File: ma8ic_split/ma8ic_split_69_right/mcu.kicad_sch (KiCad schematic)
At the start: 26 parts, among them J1 USB_C_Receptacle, J2 MJ-4PP-9, SW1 SW_PUSH, U1 ATMEGA32U4, X1 CSTNE16M0V530000R0

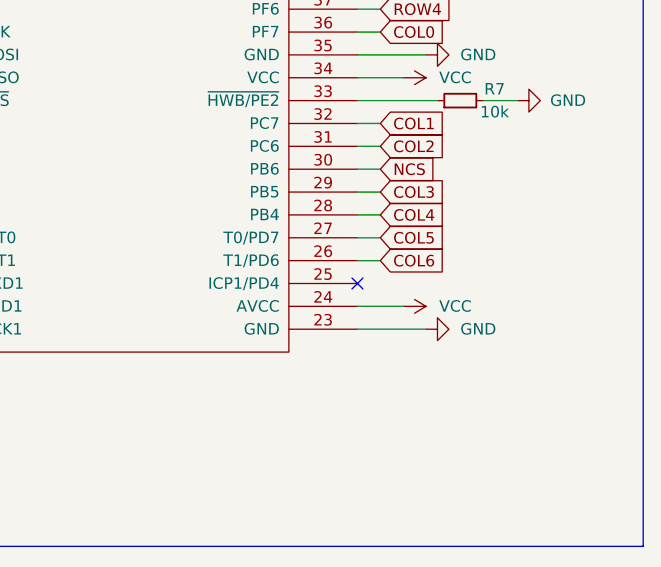
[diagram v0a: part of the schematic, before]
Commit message: update
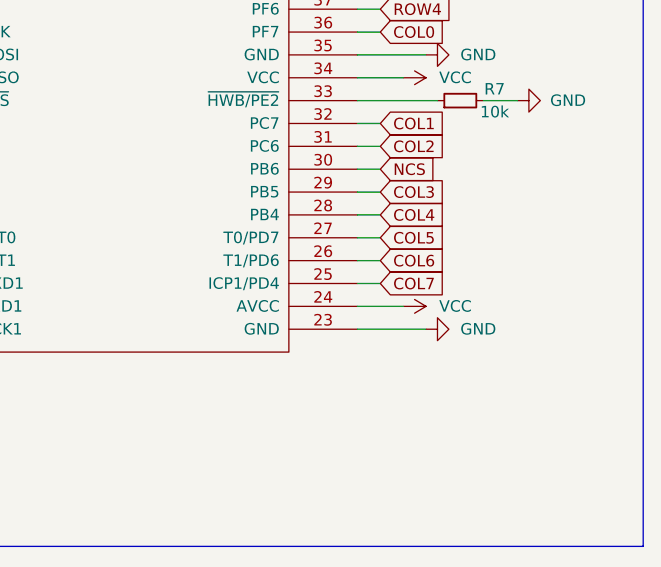
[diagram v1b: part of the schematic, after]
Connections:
- net COL7: now reaches U1.25 (ICP1/PD4)
- no-connect marks 14 -> 13
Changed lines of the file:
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@@
   (no_connect (at 52.07 66.04))
   (no_connect (at 50.8 173.99))
-  (no_connect (at 209.55 81.28))
   (no_connect (at 154.94 60.96))
   (no_connect (at 154.94 33.02))
@@
     (stroke (width 0) (type default) (color 0 0 0 0))
   )
+  (wire (pts (xy 209.55 81.28) (xy 212.09 81.28))
+    (stroke (width 0) (type default) (color 0 0 0 0))
+  )
   (wire (pts (xy 95.25 175.26) (xy 95.25 177.8))
     (stroke (width 0) (type default) (color 0 0 0 0))
@@
     (effects (font (size 1.27 1.27)) (justify right bottom))
   )
+  (global_label "COL7" (shape input) (at 212.09 81.28 0) (fields_autoplaced)
+    (effects (font (size 1.27 1.27)) (justify left))
+    (property "Intersheet References" "${INTERSHEET_REFS}" (id 0) (at 219.3412 81.2006 0)
+      (effects (font (size 1.27 1.27)) (justify left) hide)
+    )
+  )
   (global_label "ROW2" (shape input) (at 212.09 45.72 0) (fields_autoplaced)

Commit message: update
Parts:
- C1, C3, C4, C5, C6: LCSC (none) -> C14663
- C2: LCSC (none) -> C15849
- C7: LCSC (none) -> C19666
- D1, D2: LCSC (none) -> C84263
- D3: LCSC (none) -> C84266
- J1: LCSC (none) -> C778726
- R1, R2: LCSC (none) -> C23186
- R10, R11, R6, R7: LCSC (none) -> C25804
- R3, R4: LCSC (none) -> C23345
- R5, R8, R9: LCSC (none) -> C21190
- U1: footprint ma8ic_split_69:TQFP-44_10x10mm_P0.8mm -> ma8ic_split_69:QFN-44-1EP_7x7mm_P0.5mm_EP5.2x5.2mm; LCSC (none) -> C112161
- X1: LCSC (none) -> C341521
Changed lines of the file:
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@@
+      (effects (font (size 1.27 1.27)) hide)
+    )
+    (property "LCSC" "C14663" (id 4) (at 25.4 134.62 0)
       (effects (font (size 1.27 1.27)) hide)
     )
@@
       (effects (font (size 1.27 1.27)) hide)
     )
+    (property "LCSC" "C25804" (id 4) (at 138.43 58.42 0)
+      (effects (font (size 1.27 1.27)) hide)
+    )
     (pin "1")
     (pin "2")
@@
       (effects (font (size 1.27 1.27)) hide)
     )
+    (property "LCSC" "C19666" (id 4) (at 50.8 134.62 0)
+      (effects (font (size 1.27 1.27)) hide)
+    )
     (pin "1")
     (pin "2")
@@
     )
     (property "Datasheet" "~" (id 3) (at 220.98 38.1 0)
+      (effects (font (size 1.27 1.27)) hide)
+    )
+    (property "LCSC" "C14663" (id 4) (at 220.98 38.1 0)
       (effects (font (size 1.27 1.27)) hide)
     )
@@
       (effects (font (size 1.27 1.27)) (justify bottom) hide)
     )
+    (property "LCSC" "C341521" (id 8) (at 138.43 133.35 0)
+      (effects (font (size 1.27 1.27)) hide)
+    )
     (pin "1")
     (pin "2")
@@
       (effects (font (size 1.27 1.27)) hide)
     )
+    (property "LCSC" "C21190" (id 4) (at 137.16 86.36 0)
+      (effects (font (size 1.27 1.27)) hide)
+    )
     (pin "1")
     (pin "2")
@@
       (effects (font (size 1.27 1.27)) hide)
     )
+    (property "LCSC" "C23186" (id 4) (at 59.69 30.48 0)
+      (effects (font (size 1.27 1.27)) hide)
+    )
     (pin "1")
     (pin "2")
@@
       (effects (font (size 1.27 1.27)) hide)
     )
+    (property "LCSC" "C23186" (id 4) (at 59.69 33.02 0)
+      (effects (font (size 1.27 1.27)) hide)
+    )
     (pin "1")
     (pin "2")
@@
       (effects (font (size 1.27 1.27)) hide)
     )
+    (property "LCSC" "C25804" (id 4) (at 220.98 60.96 0)
+      (effects (font (size 1.27 1.27)) hide)
+    )
     (pin "1")
     (pin "2")
@@
     )
     (property "Datasheet" "https://www.usb.org/sites/default/files/documents/usb_type-c.zip" (id 3) (at 40.64 50.8 0)
+      (effects (font (size 1.27 1.27)) hide)
+    )
+    (property "LCSC" "C778726" (id 4) (at 36.83 50.8 0)
       (effects (font (size 1.27 1.27)) hide)
     )
@@
       (effects (font (size 1.27 1.27)) hide)
     )
+    (property "LCSC" "C14663" (id 4) (at 38.1 134.62 0)
+      (effects (font (size 1.27 1.27)) hide)
+    )
     (pin "1")
     (pin "2")
@@
     )
     (property "Datasheet" "~" (id 3) (at 44.45 134.62 0)
+      (effects (font (size 1.27 1.27)) hide)
+    )
+    (property "LCSC" "C14663" (id 4) (at 44.45 134.62 0)
       (effects (font (size 1.27 1.27)) hide)
     )
@@
       (effects (font (size 1.27 1.27)) hide)
     )
+    (property "LCSC" "C23345" (id 4) (at 59.69 43.18 0)
+      (effects (font (size 1.27 1.27)) hide)
+    )
     (pin "1")
     (pin "2")
@@
       (effects (font (size 1.27 1.27)) hide)
     )
+    (property "LCSC" "C21190" (id 4) (at 82.55 137.16 0)
+      (effects (font (size 1.27 1.27)) hide)
+    )
     (pin "1")
     (pin "2")
@@
       (effects (font (size 1.27 1.27)) hide)
     )
+    (property "LCSC" "C14663" (id 4) (at 31.75 134.62 0)
+      (effects (font (size 1.27 1.27)) hide)
+    )
     (pin "1")
     (pin "2")
@@
       (effects (font (size 1.27 1.27)) hide)
     )
+    (property "LCSC" "C84263" (id 4) (at 128.27 50.8 0)
+      (effects (font (size 1.27 1.27)) hide)
+    )
     (pin "1")
     (pin "2")
@@
       (effects (font (size 1.27 1.27)) hide)
     )
+    (property "LCSC" "C23345" (id 4) (at 59.69 40.64 0)
+      (effects (font (size 1.27 1.27)) hide)
+    )
     (pin "1")
     (pin "2")
@@
       (effects (font (size 1.27 1.27)) hide)
     )
+    (property "LCSC" "C25804" (id 4) (at 95.25 180.34 0)
+      (effects (font (size 1.27 1.27)) hide)
+    )
     (pin "1")
     (pin "2")
@@
       (effects (font (size 1.27 1.27)) hide)
     )
+    (property "LCSC" "C25804" (id 4) (at 88.9 180.34 0)
+      (effects (font (size 1.27 1.27)) hide)
+    )
     (pin "1")
     (pin "2")
@@
     )
     (property "Datasheet" "~" (id 3) (at 148.59 45.72 0)
+      (effects (font (size 1.27 1.27)) hide)
+    )
+    (property "LCSC" "C15849" (id 4) (at 148.59 45.72 0)
       (effects (font (size 1.27 1.27)) hide)
     )
@@
       (effects (font (size 1.27 1.27)) hide)
     )
+    (property "LCSC" "C84266" (id 4) (at 91.44 137.16 0)
+      (effects (font (size 1.27 1.27)) hide)
+    )
     (pin "1")
     (pin "2")
@@
       (effects (font (size 1.27 1.27)) hide)
     )
+    (property "LCSC" "C84263" (id 4) (at 128.27 86.36 0)
+      (effects (font (size 1.27 1.27)) hide)
+    )
     (pin "1")
     (pin "2")
@@
       (effects (font (size 1.524 1.524)))
     )
-    (property "Footprint" "ma8ic_split_69:TQFP-44_10x10mm_P0.8mm" (id 2) (at 181.61 59.69 0)
+    (property "Footprint" "ma8ic_split_69:QFN-44-1EP_7x7mm_P0.5mm_EP5.2x5.2mm" (id 2) (at 181.61 59.69 0)
       (effects (font (size 1.524 1.524)) hide)
     )
     (property "Datasheet" "" (id 3) (at 181.61 59.69 0)
       (effects (font (size 1.524 1.524)) hide)
+    )
+    (property "LCSC" "C112161" (id 4) (at 181.61 59.69 0)
+      (effects (font (size 1.27 1.27)) hide)
     )
     (pin "1")
@@
       (effects (font (size 1.27 1.27)) hide)
     )
+    (property "LCSC" "C21190" (id 4) (at 137.16 50.8 0)
+      (effects (font (size 1.27 1.27)) hide)
+    )
